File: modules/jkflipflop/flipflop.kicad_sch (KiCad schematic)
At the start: 1 part

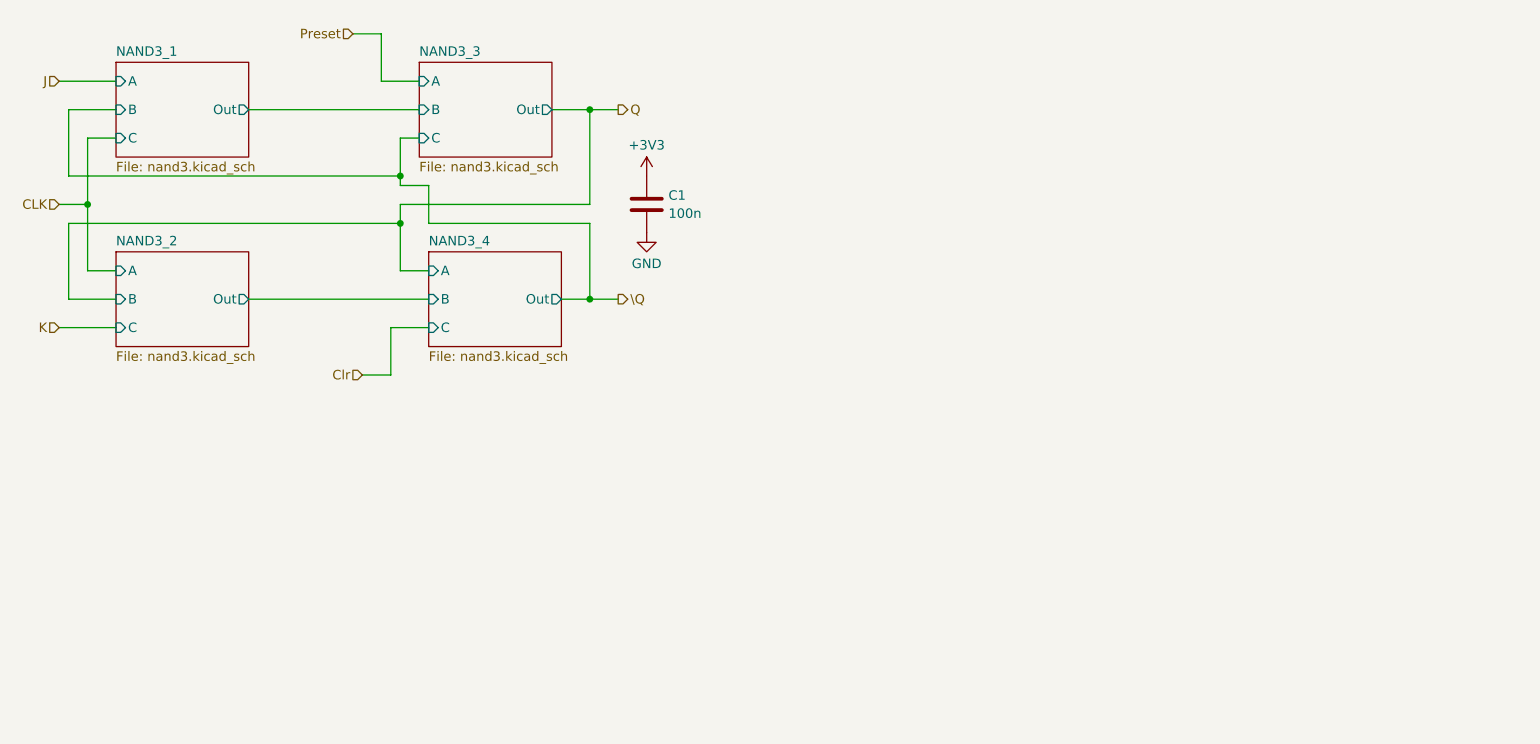
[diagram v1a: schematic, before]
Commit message: flipflop wip
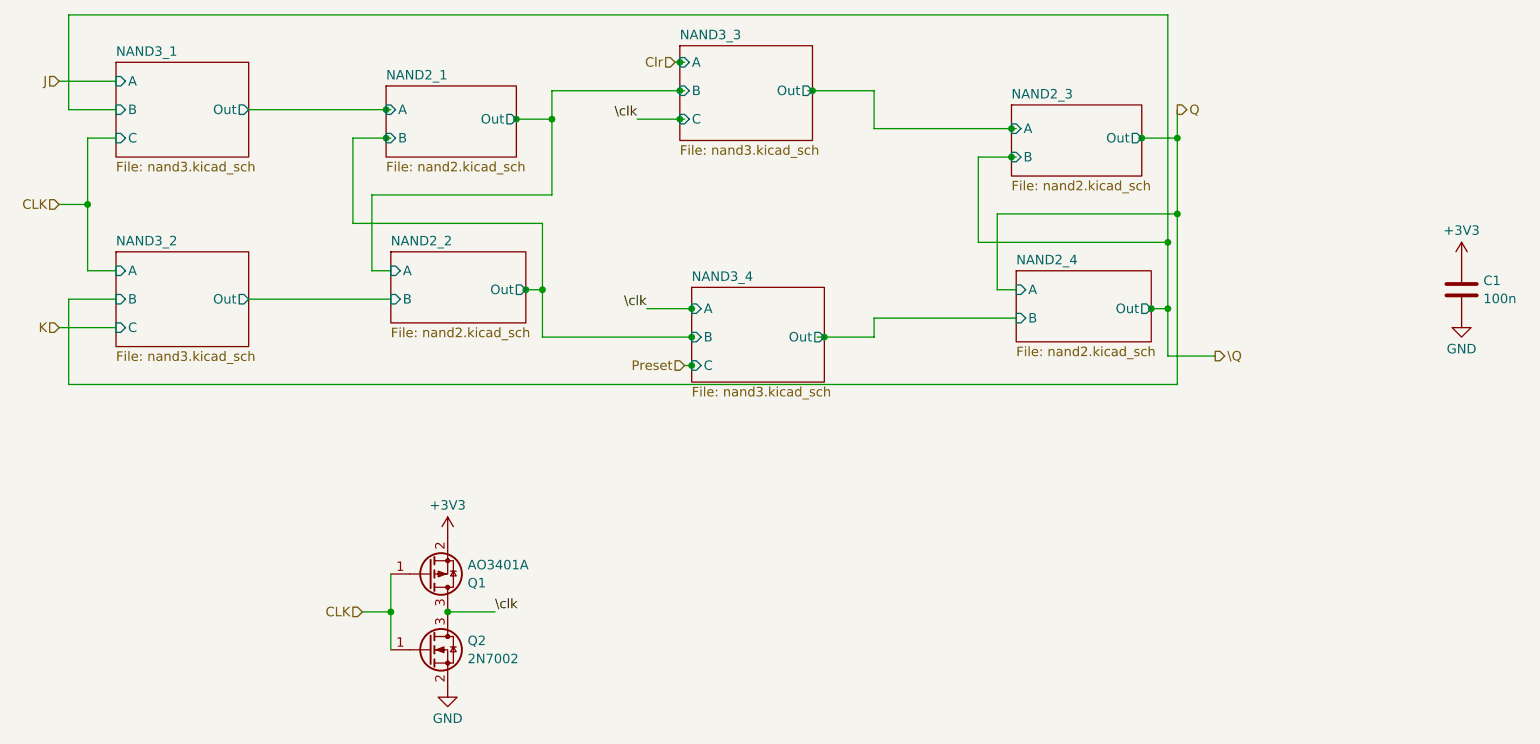
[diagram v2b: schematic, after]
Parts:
- added Q1: AO3401A, Package_TO_SOT_SMD:SOT-23, symbol Transistor_FET:DMP3099L
- added Q2: 2N7002, Package_TO_SOT_SMD:SOT-23, symbol Transistor_FET:2N7002
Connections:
- net +3V3: now also Q1.2 (S)
- net CLK: now also Q1.1 (G), Q2.1 (G)
- net GND: now also Q2.2 (S)
- new net \clk: Q1.3 (D), Q2.3 (D)
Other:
- added sheet NAND2_1 (nand2.kicad_sch)
- added sheet NAND2_2 (nand2.kicad_sch)
- added sheet NAND2_3 (nand2.kicad_sch)
- added sheet NAND2_4 (nand2.kicad_sch)
- moved on the sheet: C1
